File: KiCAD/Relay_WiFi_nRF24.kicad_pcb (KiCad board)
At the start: 2 copper layers, 50.8 x 50.8 mm, 15 parts, among them IC1 MOC3061M, P1 CONN_4, P2 CONN_4, P3 CONN_01X04, U1 ESP8266-ESP-03, U2 NCP1117ST33T3G, U3 NRF24L01P_SMD, U4 TRIAC

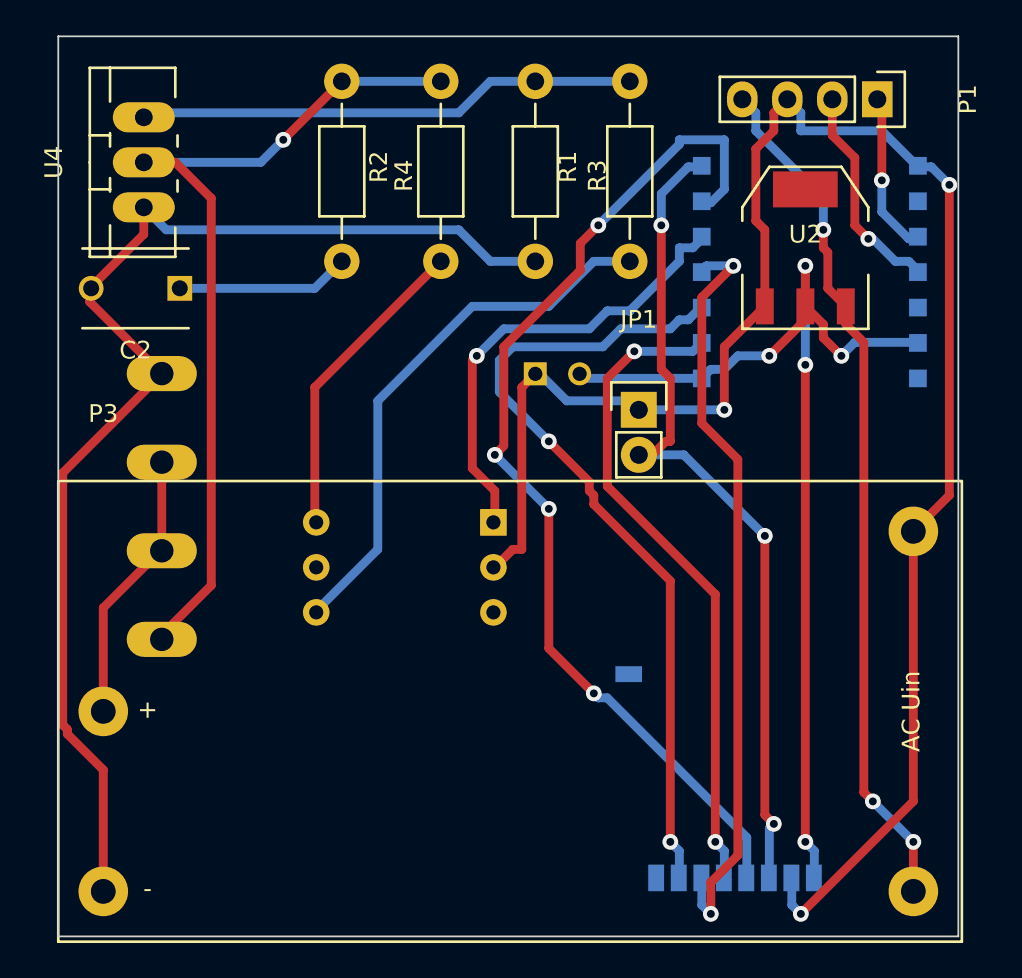
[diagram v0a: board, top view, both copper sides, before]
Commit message: Мелкие изменения
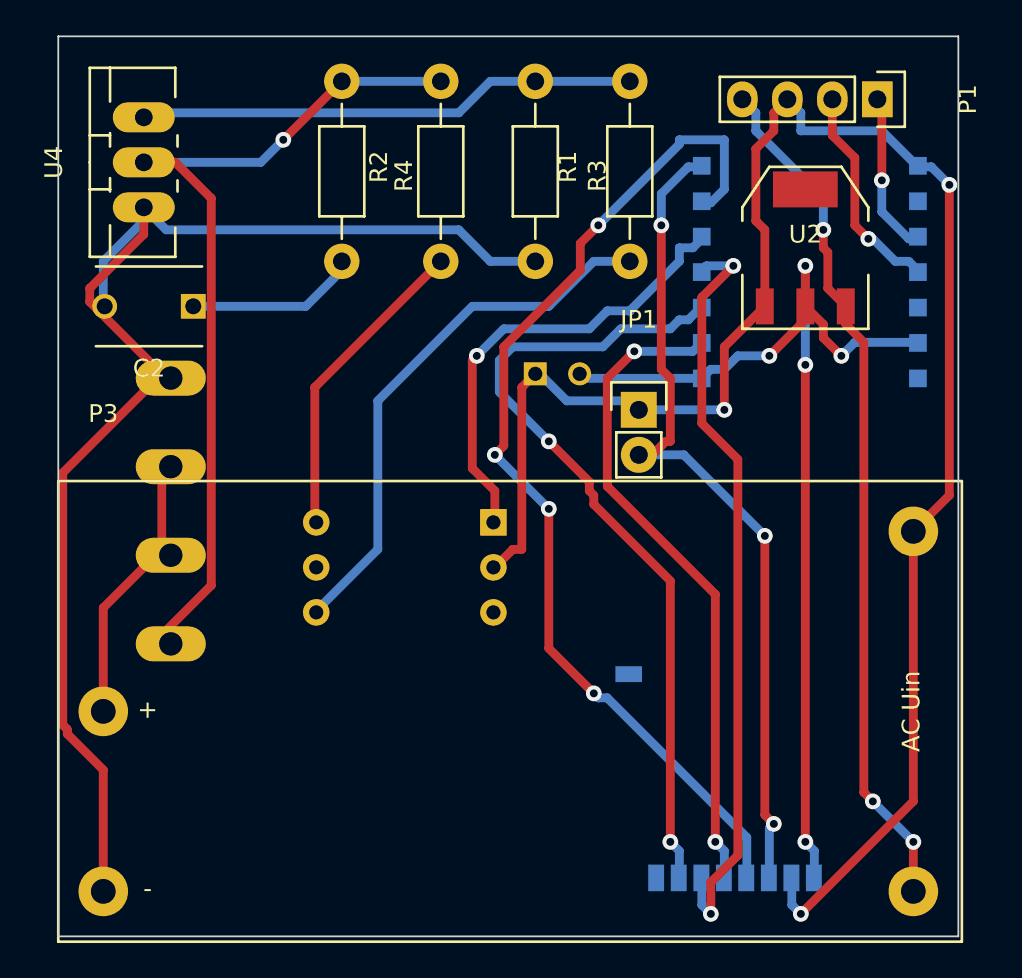
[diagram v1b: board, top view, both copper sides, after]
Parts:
- moved C2 1.27 mm to (171.4, 133.3)
- moved P2 0.57 mm to (170.2, 152.4)
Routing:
- net Net-(C2-Pad2): track 68.4 -> 75.0 mm
- net Net-(C2-Pad1): track 9.78 -> 10.5 mm
